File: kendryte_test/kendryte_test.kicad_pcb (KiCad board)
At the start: 2 copper layers, 2 parts, among them J1 Conn_01x08_Male, U1 K210_POWER

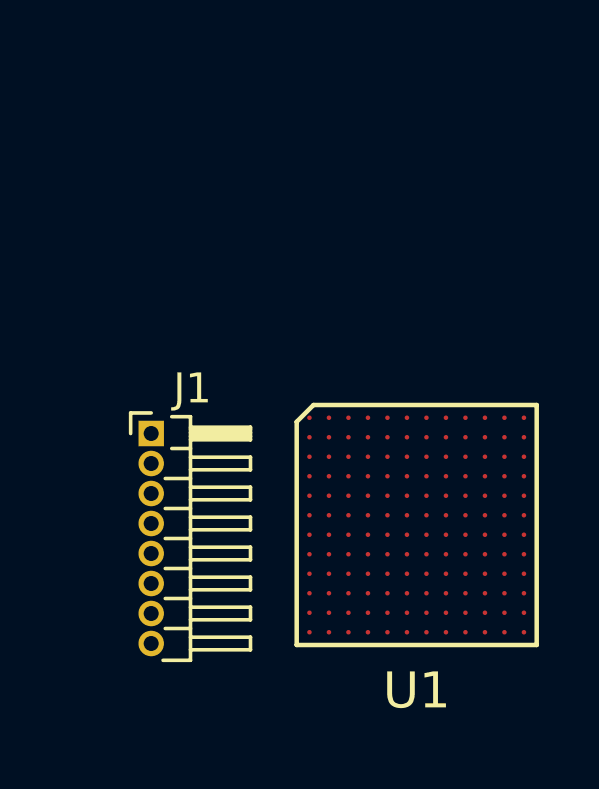
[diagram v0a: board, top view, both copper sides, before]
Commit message: K210 more work
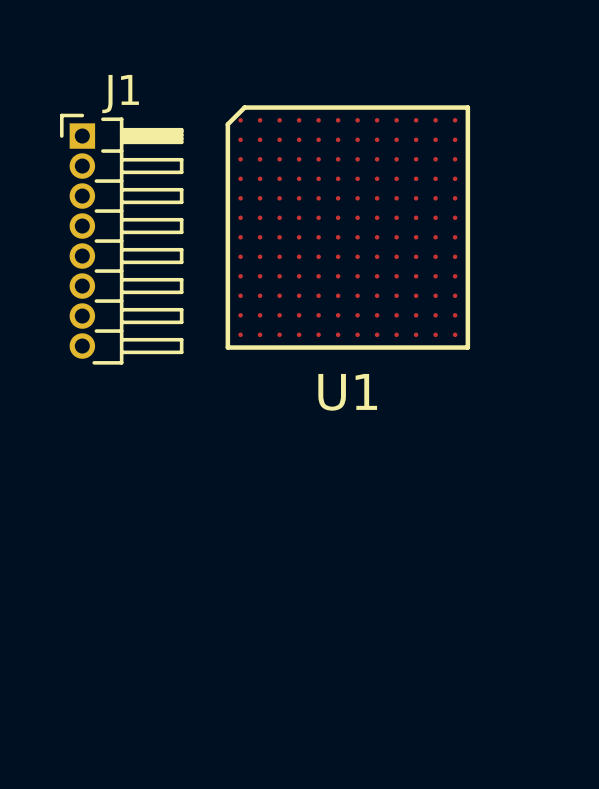
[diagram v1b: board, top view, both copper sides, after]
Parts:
- U1: value K210_POWER -> K210
- moved U1 10.2 mm to (190.5, -40.1)
- moved J1 10.2 mm to (181.6, -43.2)
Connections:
- U1 pad C10: (no net) -> Earth
- U1 pad C3: (no net) -> Earth
- U1 pad C4: (no net) -> Earth
- U1 pad C5: (no net) -> Net-(U1-PadC5)
- U1 pad C6: (no net) -> Earth
- U1 pad C7: (no net) -> Net-(U1-PadC5)
- U1 pad C8: (no net) -> Net-(U1-PadC5)
- U1 pad C9: (no net) -> Earth
- U1 pad D10: Net-(J1-Pad3) -> Net-(U1-PadD10)
- U1 pad D3: (no net) -> Net-(U1-PadD3)
- U1 pad D4: (no net) -> /VCORE
- U1 pad D5: (no net) -> Earth
- U1 pad D6: (no net) -> /VCORE
- U1 pad D7: (no net) -> Earth
- U1 pad D8: (no net) -> Earth
- U1 pad D9: (no net) -> /VCORE
- U1 pad E10: (no net) -> Earth
- U1 pad E3: (no net) -> Earth
- U1 pad E4: (no net) -> Earth
- U1 pad E5: (no net) -> Earth
- U1 pad E6: (no net) -> Earth
- U1 pad E7: (no net) -> /VCORE
- U1 pad E8: (no net) -> Earth
- U1 pad E9: (no net) -> /VCORE
- U1 pad F10: (no net) -> Earth
- U1 pad F3: (no net) -> Net-(U1-PadD3)
- U1 pad F4: (no net) -> /VCORE
- U1 pad F5: (no net) -> Earth
- U1 pad F6: (no net) -> /VCORE
- U1 pad F7: (no net) -> Earth
- U1 pad F8: (no net) -> Earth
- U1 pad F9: (no net) -> Earth
- U1 pad G10: Net-(J1-Pad2) -> Net-(U1-PadD10)
- U1 pad G3: (no net) -> Earth
- U1 pad G4: (no net) -> Earth
- U1 pad G5: (no net) -> Earth
- U1 pad G6: (no net) -> Earth
- U1 pad G7: (no net) -> /VCORE
- U1 pad G8: (no net) -> Earth
- U1 pad G9: (no net) -> /VCORE
- U1 pad H10: Net-(J1-Pad1) -> Net-(U1-PadD10)
- U1 pad H2: (no net) -> Earth
- U1 pad H3: (no net) -> Net-(U1-PadH3)
- U1 pad H4: (no net) -> /VCORE
- U1 pad H5: (no net) -> Earth
- U1 pad H6: (no net) -> /VCORE
- U1 pad H7: (no net) -> Earth
- U1 pad H8: (no net) -> Earth
- U1 pad H9: (no net) -> Earth
- U1 pad J10: (no net) -> Earth
- U1 pad J2: (no net) -> Earth
- U1 pad J3: (no net) -> Net-(U1-PadJ3)
- U1 pad J4: (no net) -> Earth
- U1 pad J5: (no net) -> /VCORE
- U1 pad J6: (no net) -> Earth
- U1 pad J7: (no net) -> /VCORE
- U1 pad J8: (no net) -> Earth
- U1 pad J9: (no net) -> /VCORE
- U1 pad K10: (no net) -> Earth
- U1 pad K2: (no net) -> Earth
- U1 pad K3: (no net) -> Earth
- U1 pad K4: (no net) -> Net-(U1-PadK4)
- U1 pad K5: (no net) -> Earth
- U1 pad K6: (no net) -> Net-(U1-PadK6)
- U1 pad K7: (no net) -> Earth
- U1 pad K8: (no net) -> Net-(U1-PadK8)
- U1 pad K9: (no net) -> Earth
- U1 pad L4: (no net) -> Net-(U1-PadL4)
